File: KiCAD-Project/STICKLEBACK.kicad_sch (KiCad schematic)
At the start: 15 parts, among them J1 DE9_Pins_MountingHoles, J2 AudioJack3_SwitchTR, U1 74LS30, U2 74LS367, U3 74LS138

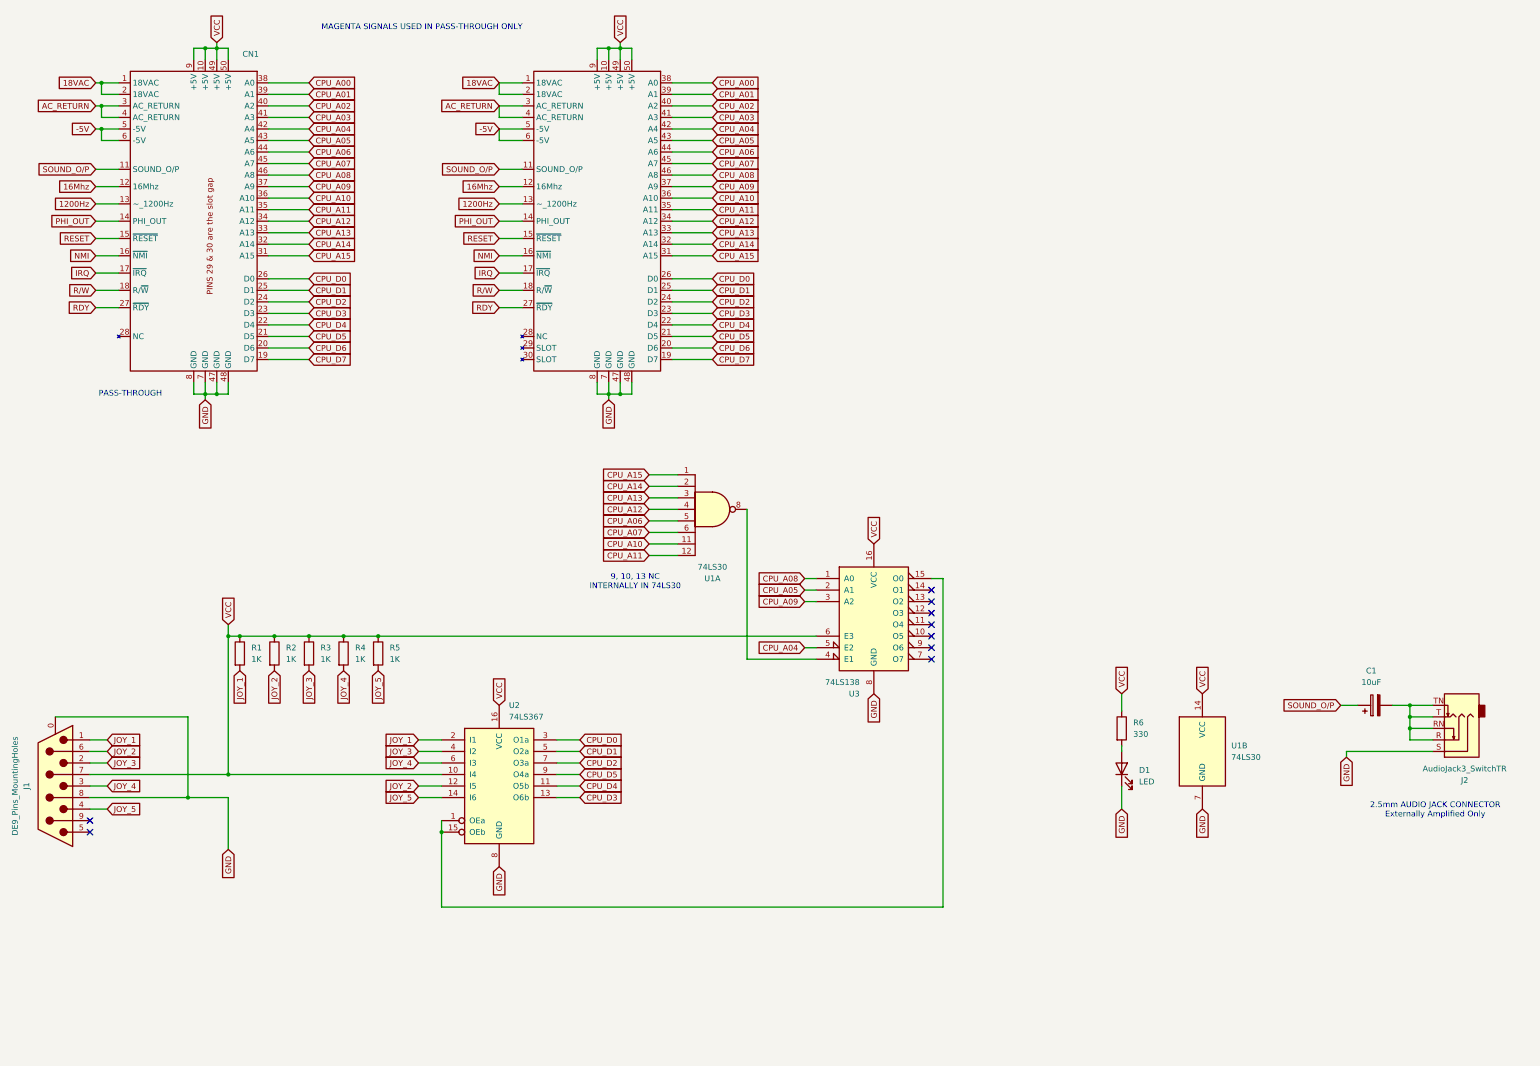
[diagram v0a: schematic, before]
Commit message: Added PDF schematics
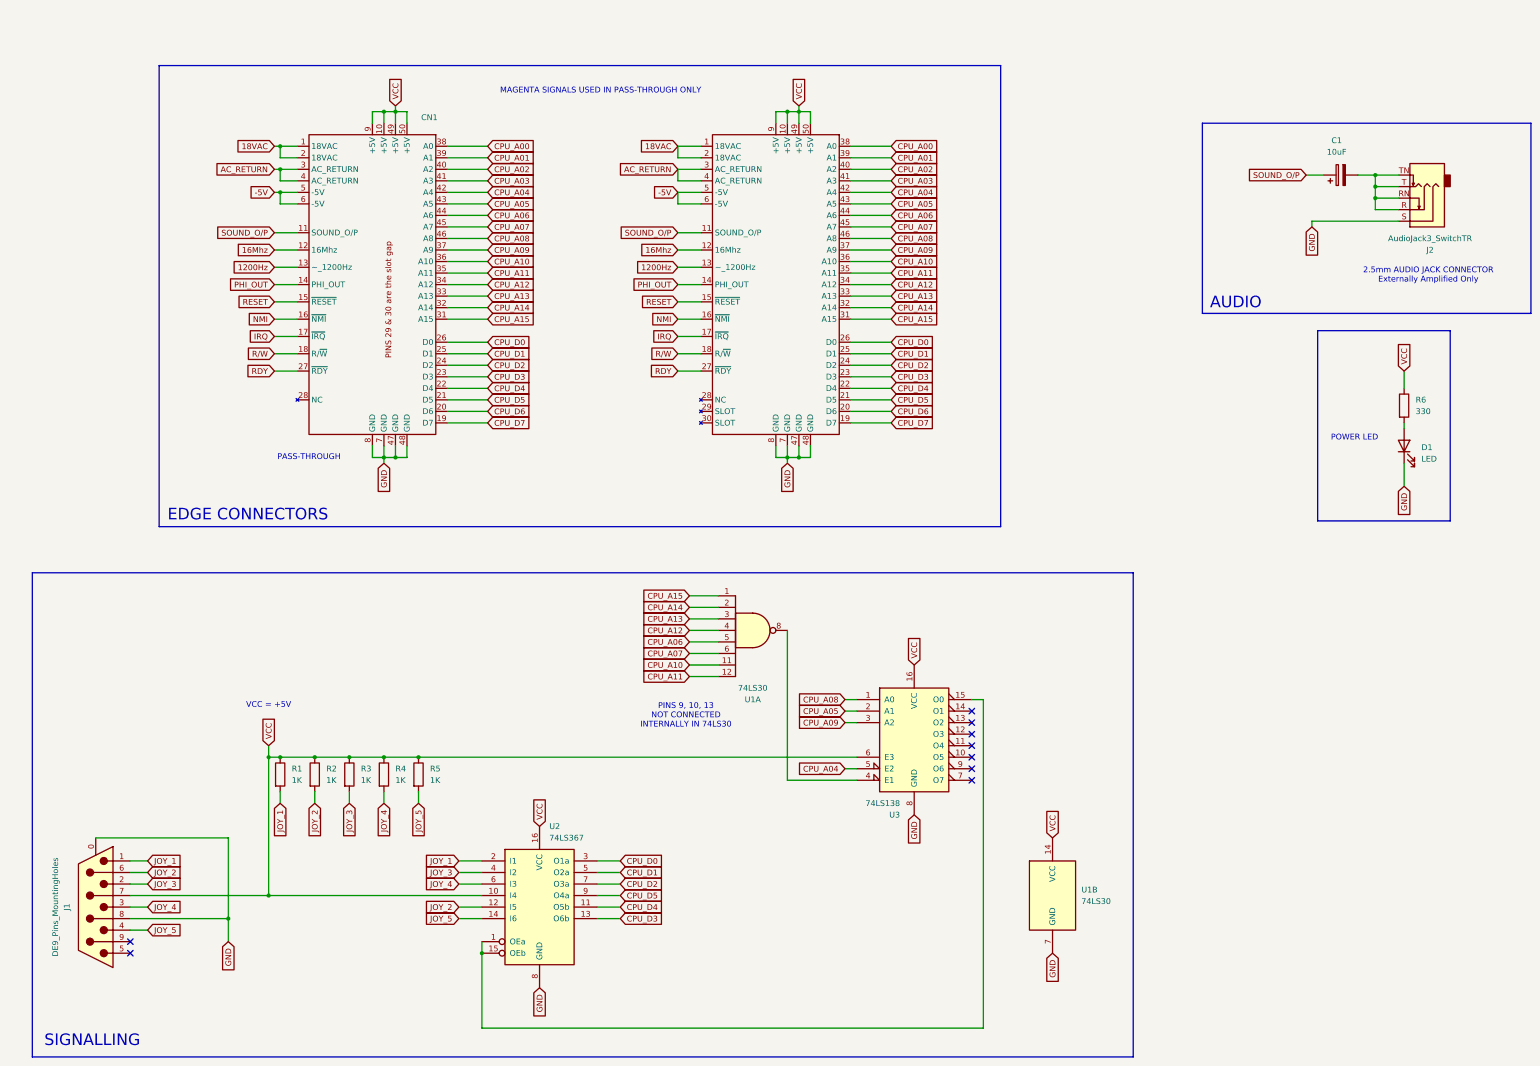
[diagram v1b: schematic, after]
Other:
- note added: "AUDIO"
- note added: "EDGE CONNECTORS"
- note added: "PINS 9, 10, 13 NOT CONNECTED INTERNALLY IN 74LS30"
- note added: "POWER LED"
- note added: "SIGNALLING"
- note added: "VCC = +5V"
- note removed: "9, 10, 13 NC INTERNALLY IN 74LS30"
- moved on the sheet: C1, CN1, D1, J1, J2, R1, R2, R3, R4, R5, R6, U1A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
